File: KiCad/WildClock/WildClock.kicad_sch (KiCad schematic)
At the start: 35 parts, among them J1 UART, Q1 CA1, Q2 CA2, Q3 CA3, Q4 CA4, Q5 CAL, SW1 ButtonUp, SW2 ButtonDown, SW3 ButtonOK, U1 ESP32-C3-MINI-1, U2 LTC-4627JR, U3 74HC595

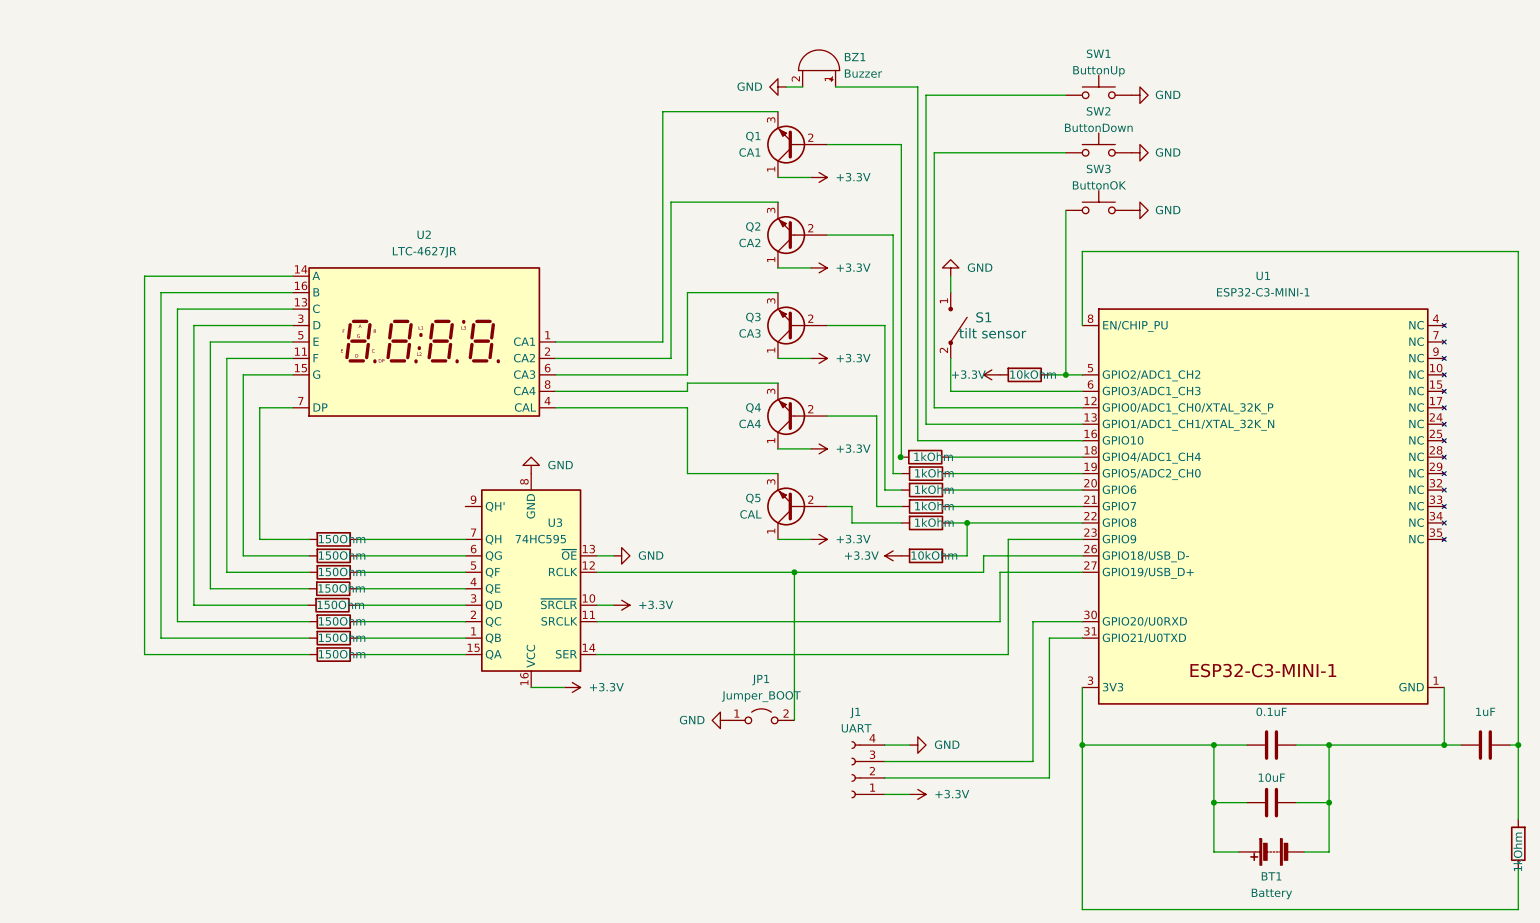
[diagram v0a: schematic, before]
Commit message: make all clearer and neu pcb
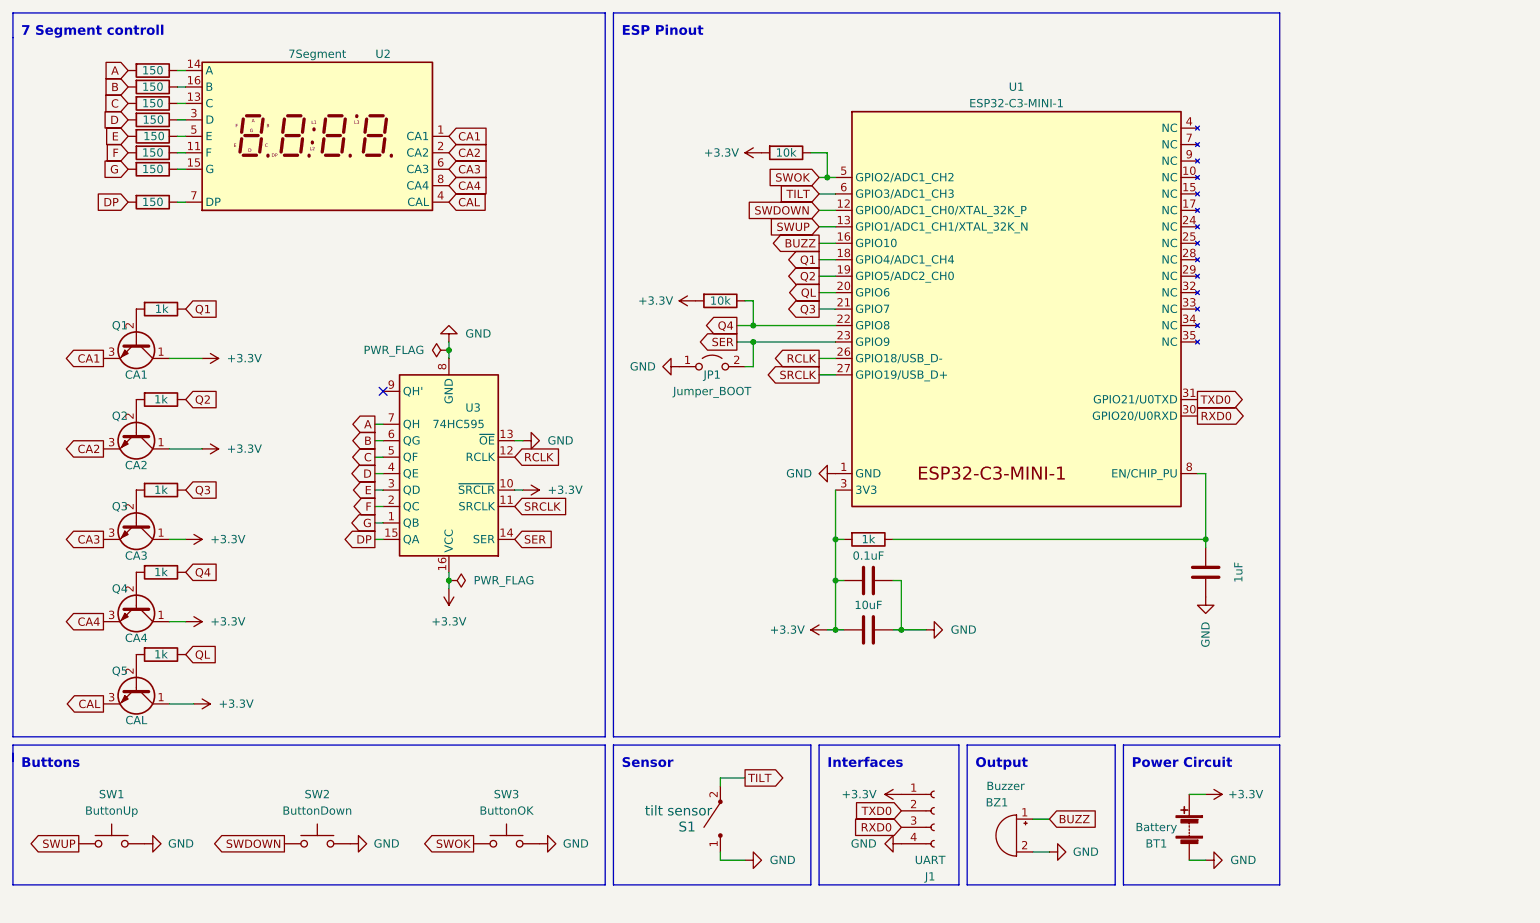
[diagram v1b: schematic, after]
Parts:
- R1, R15, R2, R3, R4, R5: value 1kOhm -> 1k
- R10, R11, R12, R13, R14, R7, R8, R9: value 150Ohm -> 150
- R16, R6: value 10kOhm -> 10k
- U2: value LTC-4627JR -> 7Segment
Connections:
- net +3.3V: now also BT1.1 (+), C1.2, C2.2, R15.2, U1.3 (3V3)
- net GND: now also BT1.2 (-), C1.1, C2.1, C3.1, U1.1 (GND), U1.2 (GND), U1.36 (GND), U1.37 (GND), U1.38 (GND), U1.39 (GND), U1.40 (GND), U1.41 (GND), U1.42 (GND), U1.43 (GND), U1.44 (GND), U1.45 (GND), U1.46 (GND), U1.47 (GND), U1.48 (GND), U1.49 (GND), U1.50 (GND), U1.51 (GND), U1.52 (GND), U1.53 (GND)
- net Q2: now reaches R2.1, U1.19 (GPIO5/ADC2_CH0)
- net BUZZ: now reaches BZ1.1 (-), U1.16 (GPIO10)
- net at R10.1: now also U2.3 (D); no longer U3.4 (QE)
- net at U2.5 (E): now also R11.1; no longer R10.2
- net CA1: now reaches Q1.3 (E), U2.1 (CA1)
- net at R7.1: now also U2.14 (A); no longer U3.7 (QH)
- net at U2.7 (DP): now also R14.1; no longer R7.2
- net at R13.1: now also U2.15 (G); no longer U3.1 (QB)
- net at U2.16 (B): now also R8.1; no longer R13.2
- net SWOK: now reaches R16.1, SW3.1, U1.5 (GPIO2/ADC1_CH2)
- net at U2.11 (F): now also R12.1; no longer R9.2
- net at U2.13 (C): now also R9.1; no longer R12.2
- net DP: now reaches R14.2
- net DP: now also U3.15 (QA); no longer U2.14 (A)
- net B: now reaches R8.2
- net B: now also U3.6 (QG); no longer U2.15 (G)
- net CA2: now reaches Q2.3 (E), U2.2 (CA2)
- net E: now reaches R11.2
- net E: now also U3.3 (QD); no longer U2.3 (D)
- net CAL: now reaches Q5.3 (E), U2.4 (CAL)
- net CA3: now reaches Q3.3 (E), U2.6 (CA3)
- net CA4: now reaches Q4.3 (E), U2.8 (CA4)
- net TXD0: now reaches J1.2 (Pin_2), U1.31 (GPIO21/U0TXD)
- net RXD0: now reaches J1.3 (Pin_3), U1.30 (GPIO20/U0RXD)
- net SRCLK: now reaches U1.27 (GPIO19/USB_D+), U3.11 (SRCLK)
- net RCLK: now reaches U1.26 (GPIO18/USB_D-), U3.12 (RCLK)
- net RCLK: no longer JP1.2 (B)
- net SER: now reaches U1.23 (GPIO9), U3.14 (SER)
- net SER: now also JP1.2 (B)
- net F: now reaches U3.2 (QC)
- net F: now also R12.2; no longer R12.1
- net C: now reaches U3.5 (QF)
- net C: now also R9.2; no longer R9.1
- net SWDOWN: now reaches SW2.1, U1.12 (GPIO0/ADC1_CH0/XTAL_32K_P)
- net SWUP: now reaches SW1.1, U1.13 (GPIO1/ADC1_CH1/XTAL_32K_N)
- net Q1: now reaches R1.1, U1.18 (GPIO4/ADC1_CH4)
- net Q3: now reaches R3.1
- net Q3: now also U1.21 (GPIO7); no longer U1.20 (GPIO6)
- net Q4: now reaches R4.1
- net Q4: now also R6.1, U1.22 (GPIO8); no longer U1.21 (GPIO7)
- net TILT: now reaches S1.2, U1.6 (GPIO3/ADC1_CH3)
- new net: C3.2, R15.1, U1.8 (EN/CHIP_PU)
- new net A: R7.2, U3.7 (QH)
- new net D: R10.2, U3.4 (QE)
- new net G: R13.2, U3.1 (QB)
- new net QL: R5.1, U1.20 (GPIO6)
- no-connect marks 0 -> 1
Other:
- note added: "7 Segment controll"
- note added: "Buttons"
- note added: "ESP Pinout"
- note added: "Interfaces"
- note added: "Output"
- note added: "Power Circuit"
- note added: "Sensor"
- moved on the sheet: BT1, BZ1, J1, JP1, Q1, Q2, Q3, Q4, Q5, S1, SW1, SW2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
